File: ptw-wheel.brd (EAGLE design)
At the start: 54 x 45 mm, 5 parts

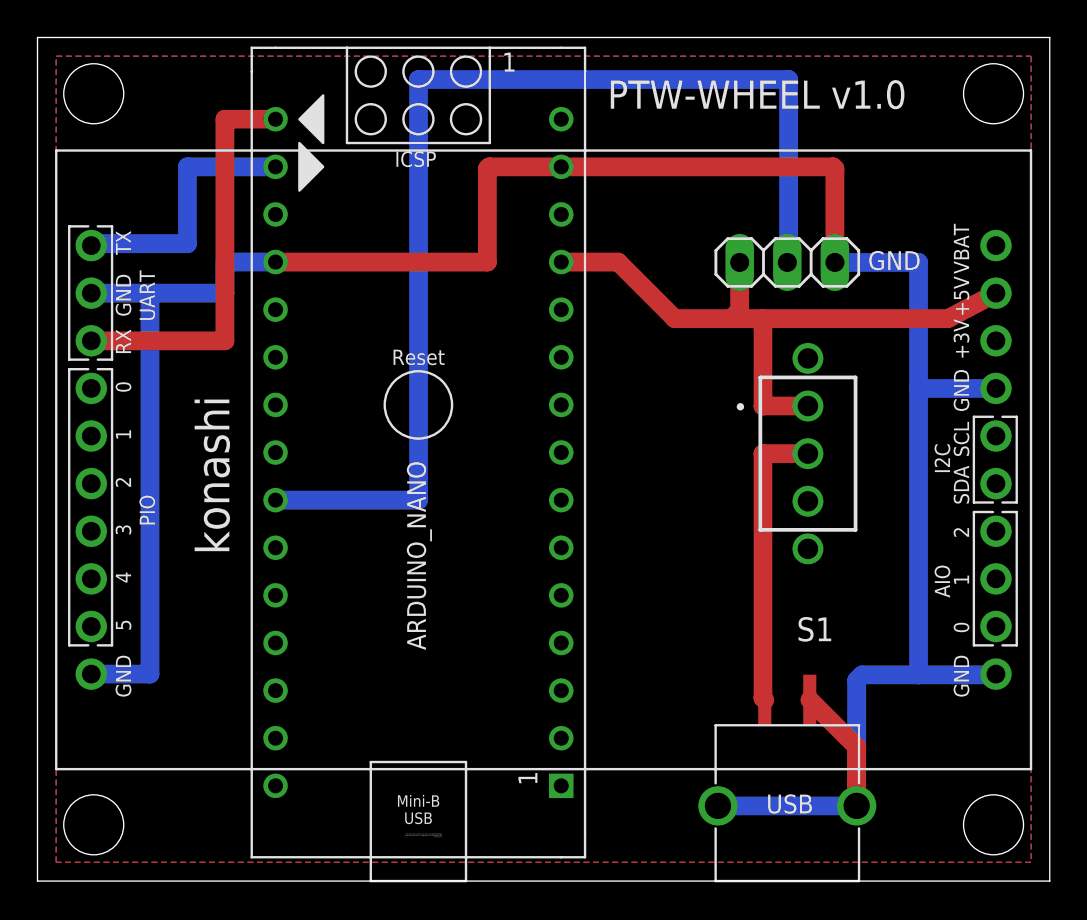
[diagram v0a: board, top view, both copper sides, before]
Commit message: 調整
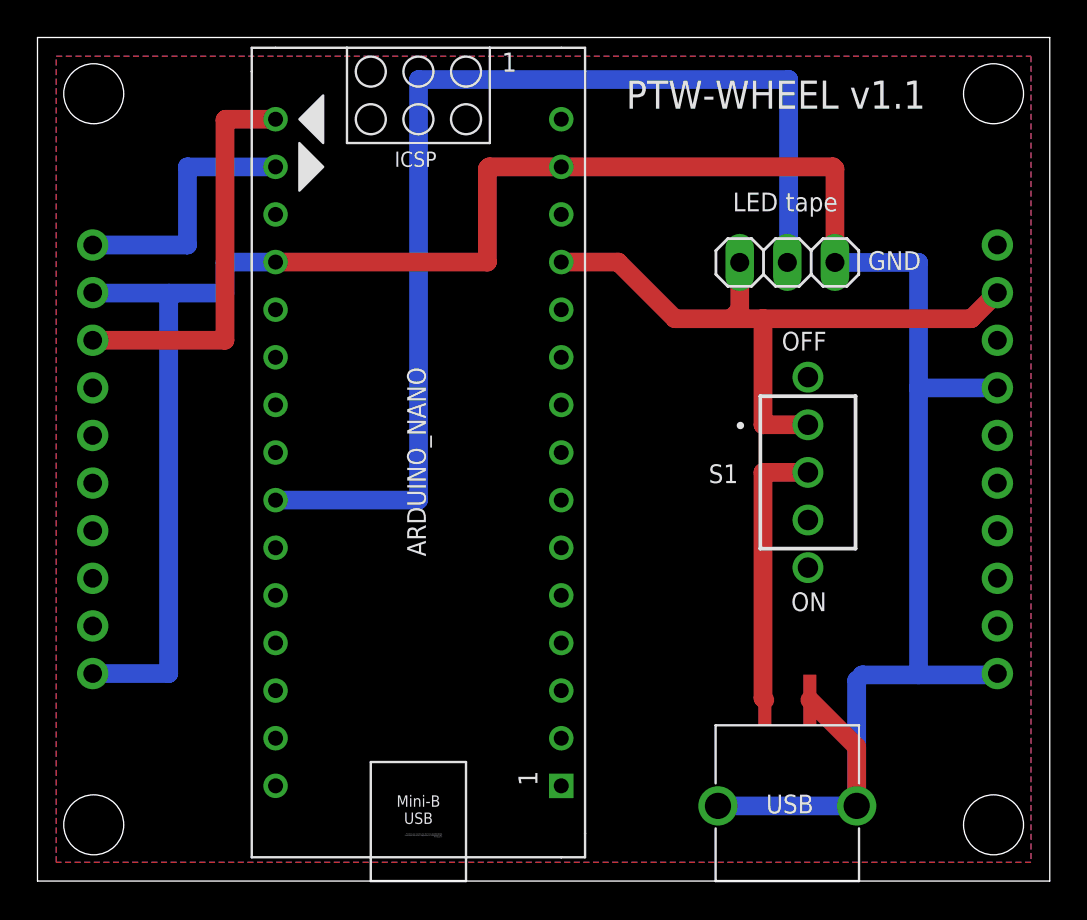
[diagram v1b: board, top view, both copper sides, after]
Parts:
- ARDUINO_NANO: device arduinoNanoV30-withoud_drill_hole:ARDUINO_NANO -> ArduinoNanoV30:ARDUINO_NANO
- JP1: value LED tapes -> LED tape
- KONASHI: device konashiv2-withoud_drill_hole:KONASHI -> konashiv2:KONASHI
- moved KONASHI 29.0 mm to (1.00, 6.00), turned to 0 degrees
- moved S1 1.00 mm to (41.1, 21.8)
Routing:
- net +5V: track 35.0 -> 36.3 mm
- net N$1: track 15.6 -> 14.6 mm
- net GND: track 133.8 -> 134.8 mm
- net N$4: track 14.6 -> 13.9 mm
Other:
- board text added: "OFF"
- board text added: "ON"
- board text added: "PTW-WHEEL v1.1"
- board text removed: "PTW-WHEEL v1.0"
